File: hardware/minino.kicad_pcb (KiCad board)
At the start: 2 copper layers, 51 x 83.5 mm, 35 parts, among them J1 OLED, J2 GPS, J3 Battery, P1 USB_C_Plug_USB2.0, Q1 DMG3415U-7, SW1 ON, SW2 RIGHT, SW3 LEFT, SW4 DOWN, SW5 UP, SW6 OK, SW7 RESET, SW8 GPIO, U1 ESP32-S3-WROOM-1U-N16, U2 MCP73831-3-OT, U3 AP2112K-3.3

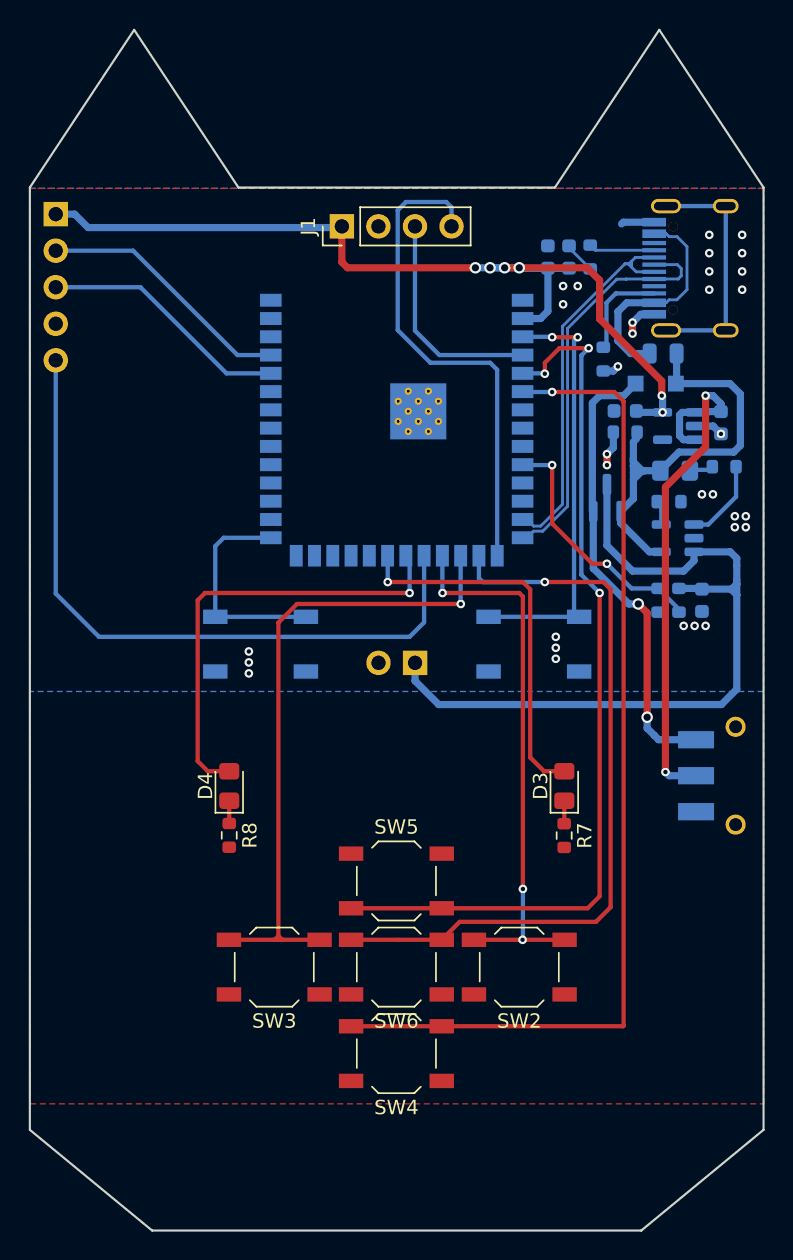
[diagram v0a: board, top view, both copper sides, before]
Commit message: Size_Adjustment
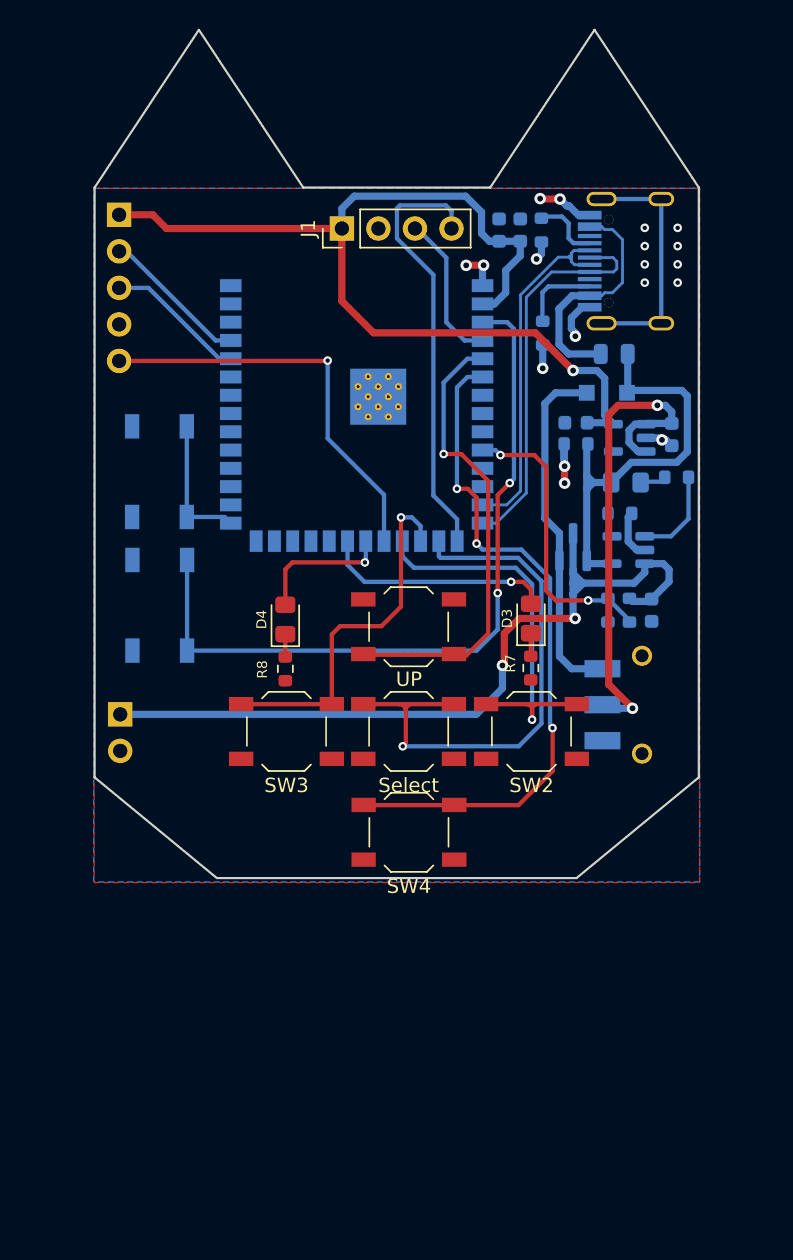
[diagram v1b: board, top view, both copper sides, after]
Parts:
- moved SW7 26.1 mm to (55.5, 76.0), turned to -90 degrees
- moved J3 20.8 mm to (52.8, 83.6), turned to 180 degrees
- moved UP 17.7 mm to (72.8, 77.5)
- moved SW2 16.4 mm to (81.4, 84.8)
- moved SW3 16.4 mm to (64.3, 84.8)
- moved Select 16.4 mm to (72.8, 84.8)
- moved SW4 15.4 mm to (72.8, 91.8)
- moved SW8 13.9 mm to (55.5, 66.8), turned to -90 degrees
- moved R8 12.2 mm to (64.3, 80.5)
- moved D4 12.2 mm to (64.3, 77.0)
- moved D3 11.9 mm to (81.3, 77.0)
- moved R7 11.9 mm to (81.3, 80.4)
- moved SW1 8.17 mm to (87.3, 83.0)
- moved R10 4.58 mm to (82.2, 57.1)
- moved P1 4.51 mm to (86.2, 52.1)
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- renumbered SW6 to Select, SW5 to UP
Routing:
- net /UP: track 62.2 -> 32.2 mm, vias 3 -> 1
- net /RST: track 29.8 -> 52.2 mm
- net /DOWN: track 69.7 -> 47.8 mm, vias 1 -> 3
- net /LED1: track 31.3 -> 9.69 mm
- net /LEFT: track 45.7 -> 25.6 mm
- net /D1: track 48.1 -> 28.7 mm, vias 0 -> 1
- net /SELECT: track 52.1 -> 39.5 mm
- net /LED2: track 26.4 -> 16.1 mm
- net /RIGHT: track 38.4 -> 28.3 mm, vias 3 -> 1
- net GND: track 12.7 -> 21.9 mm, vias 32 -> 18
- net /TX: track 18.0 -> 10.3 mm
- net /RX: track 17.4 -> 9.80 mm
- net Net-(D2-Pad1): track 31.9 -> 24.6 mm, vias 2 -> 0
- net /BOOT: track 15.3 -> 9.53 mm
- net /SCL: track 15.4 -> 10.5 mm
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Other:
- board size 51 x 83.5 mm -> 42 x 59 mm
